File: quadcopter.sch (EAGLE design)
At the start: 71 parts, among them J1 AVR_SPI_PRG_6NS, SW1 PUSHBUTTON_SMD-VERTICAL, SW2 PUSHBUTTON_SMD-VERTICAL, U1 ATMEGA128RFA1

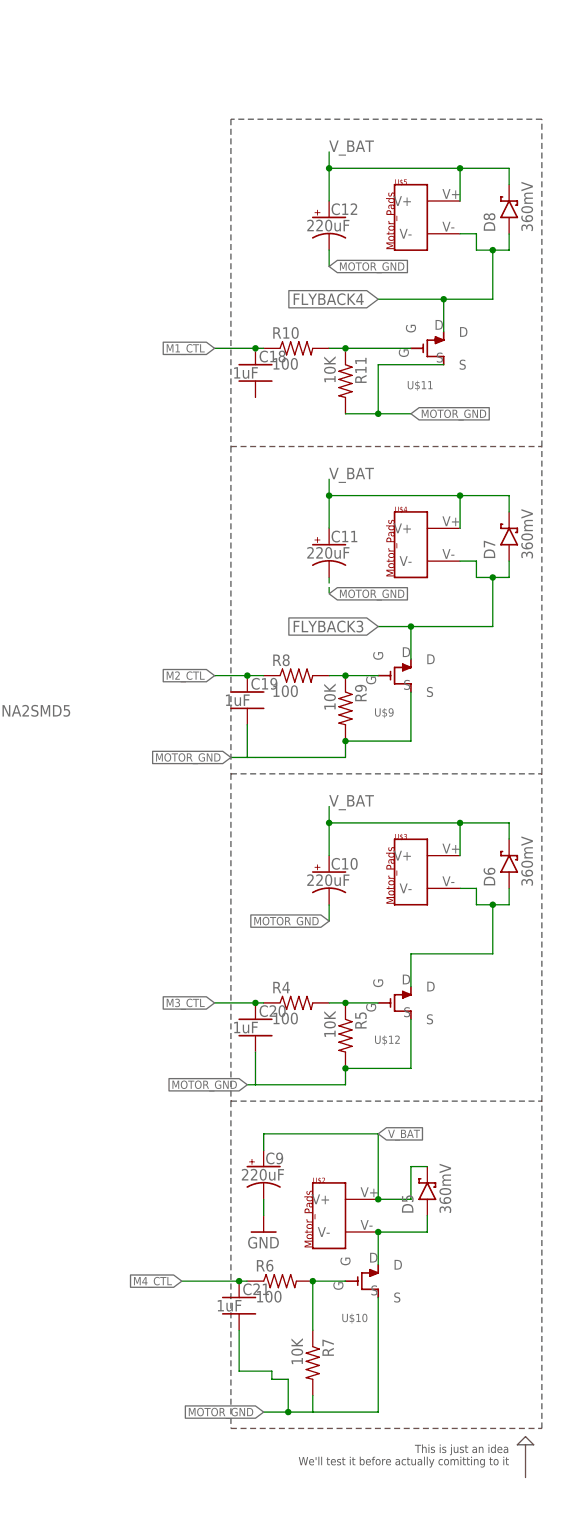
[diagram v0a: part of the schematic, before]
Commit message: started laying out basic board
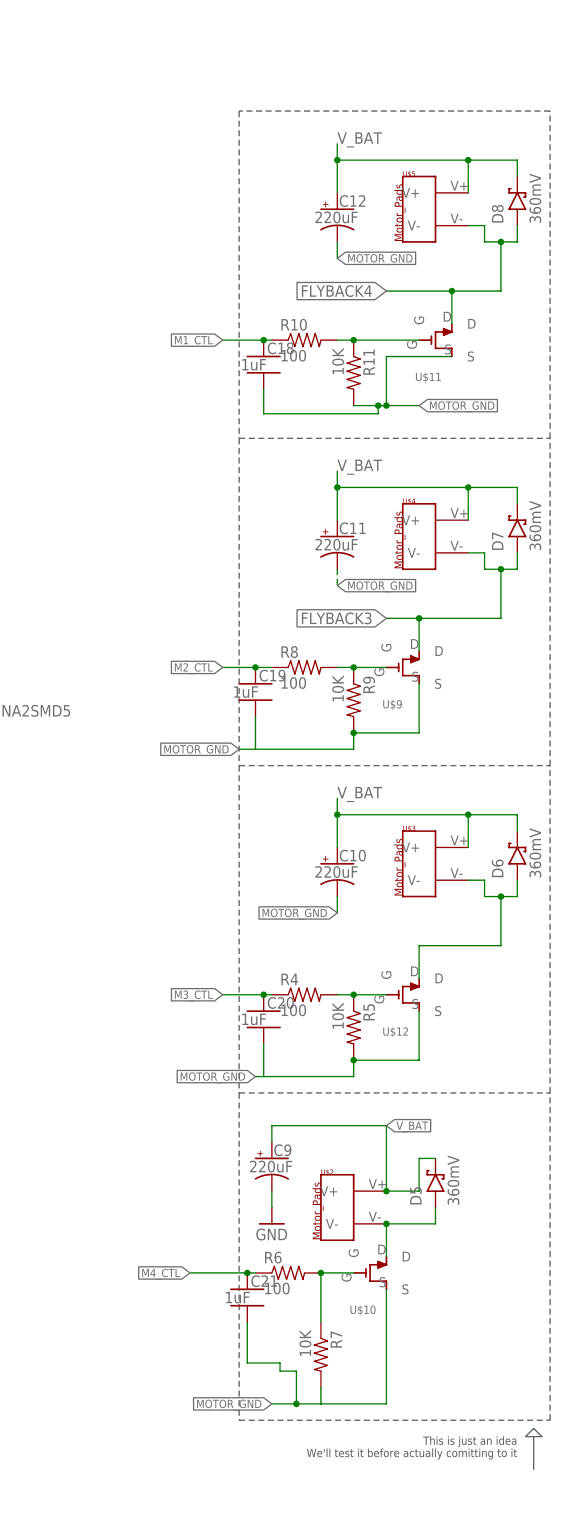
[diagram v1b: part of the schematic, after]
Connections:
- net MOTOR_GND: now also C18.2
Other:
- moved on the sheet: C10, C11, C12, C18, C19, C20, C21, C9, D5, D6, D7, D8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
